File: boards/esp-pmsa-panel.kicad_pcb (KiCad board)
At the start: 2 copper layers, 60 x 120 mm, 183 parts, among them M1 PMSA003, U1 WeMos_D1_mini_Labels, U2 BME68x, U3 OPT3001DNPT

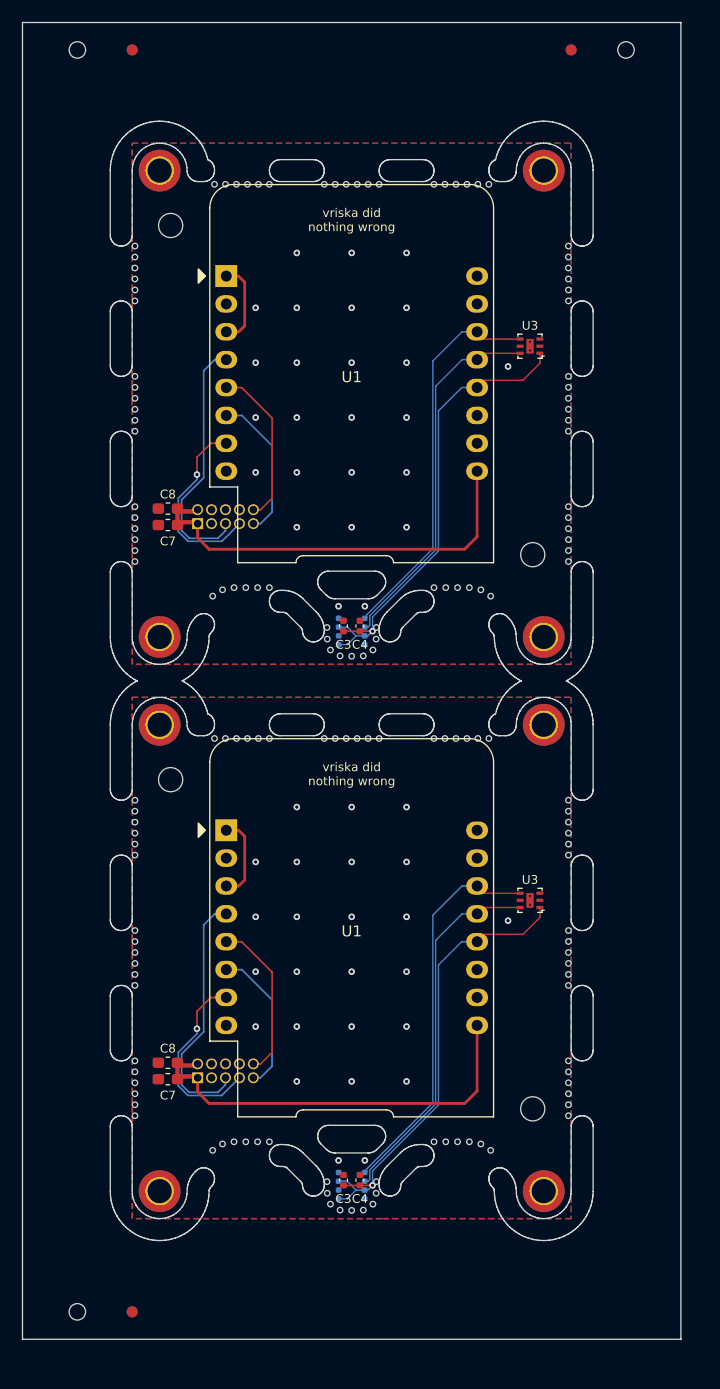
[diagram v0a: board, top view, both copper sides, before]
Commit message: Deploying to gh-pages from @ neg2led/esp-pmsa@e03a36f01e21f29b520752c6169685313d9a0f2f 🚀
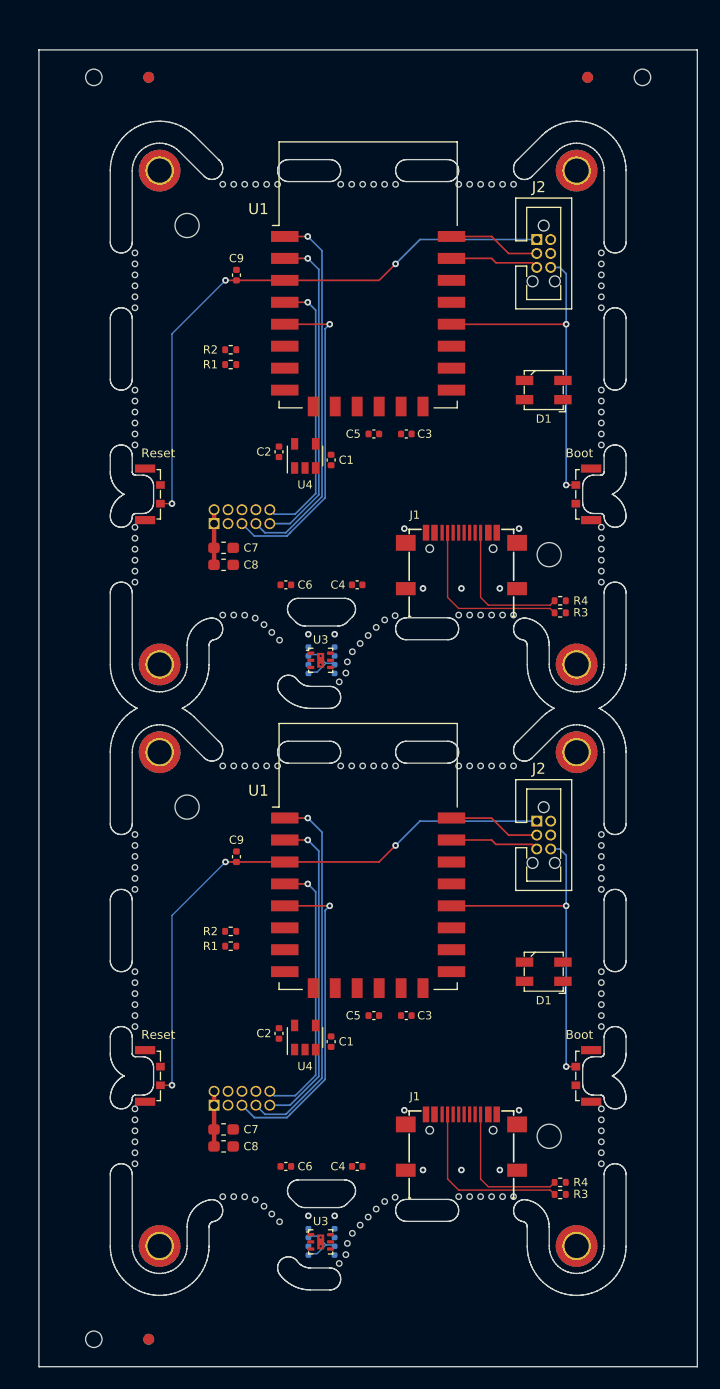
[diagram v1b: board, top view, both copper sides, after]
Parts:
- removed the C3 at (69.3, 144.5)
- removed the C3 at (69.3, 94.0)
- removed the C4 at (70.8, 144.5)
- removed the C4 at (70.8, 94.0)
- removed the C7 at (53.3, 135.3)
- removed the C7 at (53.3, 84.8)
- removed the C8 at (53.3, 133.8)
- removed the C8 at (53.3, 83.3)
- removed the H2 at (87.5, 145.5)
- removed the H2 at (87.5, 95.0)
- removed the H3 at (87.5, 103.0)
- removed the H3 at (87.5, 52.5)
- removed the H4 at (52.5, 145.5)
- removed the H4 at (52.5, 95.0)
- removed the M1 at (70.0, 123.0)
- removed the M1 at (70.0, 72.5)
- removed the REF** at (89.8, 138.6)
- removed the REF** at (89.8, 123.8)
- removed the REF** at (72.5, 104.3)
- removed the REF** at (71.5, 104.3)
- removed the REF** at (70.5, 104.3)
- removed the REF** at (69.5, 104.3)
- removed the REF** at (68.5, 104.3)
- removed the REF** at (67.5, 104.3)
- removed the REF** at (62.5, 104.3)
- removed the REF** at (61.5, 104.3)
- removed the REF** at (60.5, 104.3)
- removed the REF** at (59.5, 104.3)
- removed the REF** at (89.8, 122.8)
- removed the REF** at (58.5, 104.3)
- removed the REF** at (57.5, 104.3)
- removed the REF** at (77.5, 90.5)
- removed the REF** at (78.6, 90.5)
- removed the REF** at (79.6, 90.5)
- removed the REF** at (80.7, 90.5)
- removed the REF** at (81.8, 90.7)
- removed the REF** at (82.7, 91.3)
- removed the REF** at (67.7, 94.1)
- removed the REF** at (67.8, 95.2)
- removed the REF** at (89.8, 121.8)
- removed the REF** at (68.1, 96.2)
- removed the REF** at (68.9, 96.7)
- removed the REF** at (70.0, 96.8)
- removed the REF** at (71.1, 96.7)
- removed the REF** at (71.9, 96.2)
- removed the REF** at (72.2, 95.2)
- removed the REF** at (72.3, 94.1)
- removed the REF** at (57.3, 91.3)
- removed the REF** at (58.2, 90.7)
- removed the REF** at (59.3, 90.5)
- removed the REF** at (89.8, 114.9)
- removed the REF** at (60.4, 90.5)
- removed the REF** at (61.4, 90.5)
- removed the REF** at (62.5, 90.5)
- removed the REF** at (82.5, 53.7)
- removed the REF** at (81.5, 53.7)
- removed the REF** at (80.5, 53.7)
- removed the REF** at (79.5, 53.7)
- removed the REF** at (78.5, 53.7)
- removed the REF** at (77.5, 53.7)
- removed the REF** at (72.5, 53.7)
- removed the REF** at (89.8, 113.9)
- removed the REF** at (71.5, 53.7)
- removed the REF** at (70.5, 53.7)
- removed the REF** at (69.5, 53.7)
- removed the REF** at (68.5, 53.7)
- removed the REF** at (67.5, 53.7)
- removed the REF** at (62.5, 53.7)
- removed the REF** at (61.5, 53.7)
- removed the REF** at (60.5, 53.7)
- removed the REF** at (59.5, 53.7)
- removed the REF** at (58.5, 53.7)
- removed the REF** at (89.8, 112.9)
- removed the REF** at (57.5, 53.7)
- removed the REF** at (45.0, 156.5)
- removed the REF** at (95.0, 41.5)
- removed the REF** at (45.0, 41.5)
- removed the REF** at (50.0, 156.5) (x2)
- removed the REF** at (90.0, 41.5) (x2)
- removed the REF** at (50.0, 41.5) (x2)
- removed the REF** at (89.8, 111.9)
- removed the REF** at (89.8, 110.9)
- removed the REF** at (89.8, 109.9)
- removed the REF** at (50.2, 133.6)
- removed the REF** at (89.8, 137.6)
- removed the REF** at (50.2, 134.6)
- removed the REF** at (50.2, 135.6)
- removed the REF** at (50.2, 136.6)
- removed the REF** at (50.2, 137.6)
- removed the REF** at (50.2, 138.6)
- removed the REF** at (50.2, 121.8)
- removed the REF** at (50.2, 122.8)
- removed the REF** at (50.2, 123.8)
- removed the REF** at (50.2, 124.8)
- removed the REF** at (50.2, 125.8)
- removed the REF** at (89.8, 136.6)
- removed the REF** at (50.2, 126.8)
- removed the REF** at (50.2, 109.9)
- removed the REF** at (50.2, 110.9)
- removed the REF** at (50.2, 111.9)
- removed the REF** at (50.2, 112.9)
- removed the REF** at (50.2, 113.9)
- removed the REF** at (50.2, 114.9)
- removed the REF** at (89.8, 88.1)
- removed the REF** at (89.8, 87.1)
- removed the REF** at (89.8, 86.1)
- removed the REF** at (89.8, 135.6)
- removed the REF** at (89.8, 85.1)
- removed the REF** at (89.8, 84.1)
- removed the REF** at (89.8, 83.1)
- removed the REF** at (89.8, 76.3)
- removed the REF** at (89.8, 75.3)
- removed the REF** at (89.8, 74.3)
- removed the REF** at (89.8, 73.3)
- removed the REF** at (89.8, 72.3)
- removed the REF** at (89.8, 71.3)
- removed the REF** at (89.8, 64.4)
- removed the REF** at (89.8, 134.6)
- removed the REF** at (89.8, 63.4)
- removed the REF** at (89.8, 62.4)
- removed the REF** at (89.8, 61.4)
- removed the REF** at (89.8, 60.4)
- removed the REF** at (89.8, 59.4)
- removed the REF** at (50.2, 83.1)
- removed the REF** at (50.2, 84.1)
- removed the REF** at (50.2, 85.1)
- removed the REF** at (50.2, 86.1)
- removed the REF** at (50.2, 87.1)
- removed the REF** at (89.8, 133.6)
- removed the REF** at (50.2, 88.1)
- removed the REF** at (50.2, 71.3)
- removed the REF** at (50.2, 72.3)
- removed the REF** at (50.2, 73.3)
- removed the REF** at (50.2, 74.3)
- removed the REF** at (50.2, 75.3)
- removed the REF** at (50.2, 76.3)
- removed the REF** at (50.2, 59.4)
- removed the REF** at (50.2, 60.4)
- removed the REF** at (50.2, 61.4)
- removed the REF** at (89.8, 126.8)
- removed the REF** at (50.2, 62.4)
- removed the REF** at (50.2, 63.4)
- removed the REF** at (50.2, 64.4)
- removed the REF** at (77.5, 141.0)
- removed the REF** at (78.6, 141.0)
- removed the REF** at (79.6, 141.0)
- removed the REF** at (80.7, 141.0)
- removed the REF** at (81.8, 141.2)
- removed the REF** at (82.7, 141.8)
- removed the REF** at (67.7, 144.6)
- removed the REF** at (89.8, 125.8)
- removed the REF** at (67.8, 145.7)
- removed the REF** at (68.1, 146.7)
- removed the REF** at (68.9, 147.2)
- removed the REF** at (70.0, 147.3)
- removed the REF** at (71.1, 147.2)
- removed the REF** at (71.9, 146.7)
- removed the REF** at (72.2, 145.7)
- removed the REF** at (72.3, 144.6)
- removed the REF** at (57.3, 141.8)
- removed the REF** at (58.2, 141.2)
- removed the REF** at (89.8, 124.8)
- removed the REF** at (59.3, 141.0)
- removed the REF** at (60.4, 141.0)
- removed the REF** at (61.4, 141.0)
- removed the REF** at (62.5, 141.0)
- removed the REF** at (82.5, 104.3)
- removed the REF** at (81.5, 104.3)
- removed the REF** at (80.5, 104.3)
- removed the REF** at (79.5, 104.3)
- removed the REF** at (78.5, 104.3)
- removed the REF** at (77.5, 104.3)
- removed the U1 at (70.0, 121.5)
- removed the U1 at (70.0, 71.0)
- removed the U2 at (70.0, 145.0)
- removed the U2 at (70.0, 94.5)
- removed the U3 at (86.3, 119.0)
- removed the U3 at (86.3, 68.5)
- added C1: 10u, Capacitor_SMD:C_0402_1005Metric, F.Cu at (68.1, 131.9)
- added C1: 10u, Capacitor_SMD:C_0402_1005Metric, F.Cu at (68.1, 78.9)
- added C2: 10u, Capacitor_SMD:C_0402_1005Metric, F.Cu at (63.4, 131.1)
- added C2: 10u, Capacitor_SMD:C_0402_1005Metric, F.Cu at (63.4, 78.1)
- added C3: 1u, Capacitor_SMD:C_0402_1005Metric, F.Cu at (75.0, 129.5)
- added C3: 1u, Capacitor_SMD:C_0402_1005Metric, F.Cu at (75.0, 76.5)
- added C4: 0.1u, Capacitor_SMD:C_0402_1005Metric, F.Cu at (70.5, 143.3)
- added C4: 0.1u, Capacitor_SMD:C_0402_1005Metric, F.Cu at (70.5, 90.3)
- added C5: 1u, Capacitor_SMD:C_0402_1005Metric, F.Cu at (72.0, 129.5)
- added C5: 1u, Capacitor_SMD:C_0402_1005Metric, F.Cu at (72.0, 76.5)
- added C6: 0.1u, Capacitor_SMD:C_0402_1005Metric, F.Cu at (64.0, 143.3)
- added C6: 0.1u, Capacitor_SMD:C_0402_1005Metric, F.Cu at (64.0, 90.3)
- added C7: 10u, Capacitor_SMD:C_0603_1608Metric_Pad1.05x0.95mm_HandSolder, F.Cu at (58.3, 139.9)
- added C7: 10u, Capacitor_SMD:C_0603_1608Metric_Pad1.05x0.95mm_HandSolder, F.Cu at (58.3, 86.9)
- added C8: 10u, Capacitor_SMD:C_0603_1608Metric_Pad1.05x0.95mm_HandSolder, F.Cu at (58.3, 141.4)
- added C8: 10u, Capacitor_SMD:C_0603_1608Metric_Pad1.05x0.95mm_HandSolder, F.Cu at (58.3, 88.4)
- added C9: 0.1u, Capacitor_SMD:C_0402_1005Metric, F.Cu at (59.5, 115.0)
- added C9: 0.1u, Capacitor_SMD:C_0402_1005Metric, F.Cu at (59.5, 62.0)
- added D1: APA104-12-3535, 21-SnapEDA-zip:LED_APA104-12-3535, F.Cu at (87.5, 125.5)
- added D1: APA104-12-3535, 21-SnapEDA-zip:LED_APA104-12-3535, F.Cu at (87.5, 72.5)
- added H2: MP, MountingHole:MountingHole_2.2mm_M2_DIN965_Pad_TopBottom, F.Cu at (90.5, 150.5)
- added H2: MP, MountingHole:MountingHole_2.2mm_M2_DIN965_Pad_TopBottom, F.Cu at (90.5, 97.5)
- added H3: MP, MountingHole:MountingHole_2.2mm_M2_DIN965_Pad_TopBottom, F.Cu at (90.5, 105.5)
- added H3: MP, MountingHole:MountingHole_2.2mm_M2_DIN965_Pad_TopBottom, F.Cu at (90.5, 52.5)
- added H4: MP, MountingHole:MountingHole_2.2mm_M2_DIN965_Pad_TopBottom, F.Cu at (52.5, 150.5)
- added H4: MP, MountingHole:MountingHole_2.2mm_M2_DIN965_Pad_TopBottom, F.Cu at (52.5, 97.5)
- added J1: USB_C_Receptacle_USB2.0_304S-ACP16, 41-EasyEDA-Edits:USB-C-SMD_TYPEC-304S-ACP16, F.Cu at (80.0, 141.1)
- added J1: USB_C_Receptacle_USB2.0_304S-ACP16, 41-EasyEDA-Edits:USB-C-SMD_TYPEC-304S-ACP16, F.Cu at (80.0, 88.1)
- added J2: ESP-PROG, 11-My-Edits:TC2030_IDCBox_2x03_P1.25mm_Vertical_3D, F.Cu at (87.5, 113.1)
- added J2: ESP-PROG, 11-My-Edits:TC2030_IDCBox_2x03_P1.25mm_Vertical_3D, F.Cu at (87.5, 60.1)
- added M1: PMSA003, 12-Collected-Footprints:PMSA003, B.Cu at (71.5, 125.5)
- added M1: PMSA003, 12-Collected-Footprints:PMSA003, B.Cu at (71.5, 72.5)
- added R1: 4k7, Resistor_SMD:R_0402_1005Metric, F.Cu at (59.0, 123.2)
- added R1: 4k7, Resistor_SMD:R_0402_1005Metric, F.Cu at (59.0, 70.2)
- added R2: 4k7, Resistor_SMD:R_0402_1005Metric, F.Cu at (59.0, 121.8)
- added R2: 4k7, Resistor_SMD:R_0402_1005Metric, F.Cu at (59.0, 68.8)
- added R3: 5k1, Resistor_SMD:R_0402_1005Metric, F.Cu at (89.0, 145.8)
- added R3: 5k1, Resistor_SMD:R_0402_1005Metric, F.Cu at (89.0, 92.8)
- added R4: 5k1, Resistor_SMD:R_0402_1005Metric, F.Cu at (89.0, 144.7)
- added R4: 5k1, Resistor_SMD:R_0402_1005Metric, F.Cu at (89.0, 91.7)
- added REF**: NPTH, NPTH, F.Cu at (92.8, 143.0)
- added REF**: NPTH, NPTH, F.Cu at (92.8, 127.5)
- added REF**: NPTH, NPTH, F.Cu at (79.8, 106.8)
- added REF**: NPTH, NPTH, F.Cu at (74.0, 106.8)
- added REF**: NPTH, NPTH, F.Cu at (73.0, 106.8)
- added REF**: NPTH, NPTH, F.Cu at (72.0, 106.8)
- added REF**: NPTH, NPTH, F.Cu at (71.0, 106.8)
- added REF**: NPTH, NPTH, F.Cu at (70.0, 106.8)
- added REF**: NPTH, NPTH, F.Cu at (69.0, 106.8)
- added REF**: NPTH, NPTH, F.Cu at (63.3, 106.8)
- added REF**: NPTH, NPTH, F.Cu at (62.3, 106.8)
- added REF**: NPTH, NPTH, F.Cu at (61.3, 106.8)
- added REF**: NPTH, NPTH, F.Cu at (92.8, 126.5)
- added REF**: NPTH, NPTH, F.Cu at (60.3, 106.8)
- added REF**: NPTH, NPTH, F.Cu at (59.3, 106.8)
- added REF**: NPTH, NPTH, F.Cu at (58.3, 106.8)
- added REF**: NPTH, NPTH, F.Cu at (79.8, 93.0)
- added REF**: NPTH, NPTH, F.Cu at (80.8, 93.0)
- added REF**: NPTH, NPTH, F.Cu at (81.8, 93.0)
- added REF**: NPTH, NPTH, F.Cu at (82.8, 93.0)
- added REF**: NPTH, NPTH, F.Cu at (83.8, 93.0)
- added REF**: NPTH, NPTH, F.Cu at (84.8, 93.0)
- added REF**: NPTH, NPTH, F.Cu at (68.9, 99.1)
- added REF**: NPTH, NPTH, F.Cu at (92.8, 125.5)
- added REF**: NPTH, NPTH, F.Cu at (69.5, 98.3)
- added REF**: NPTH, NPTH, F.Cu at (69.6, 97.3)
- added REF**: NPTH, NPTH, F.Cu at (70.1, 96.3)
- added REF**: NPTH, NPTH, F.Cu at (70.8, 95.6)
- added REF**: NPTH, NPTH, F.Cu at (71.5, 94.9)
- added REF**: NPTH, NPTH, F.Cu at (72.2, 94.1)
- added REF**: NPTH, NPTH, F.Cu at (73.0, 93.4)
- added REF**: NPTH, NPTH, F.Cu at (74.0, 93.1)
- added REF**: NPTH, NPTH, F.Cu at (58.3, 93.0)
- added REF**: NPTH, NPTH, F.Cu at (59.3, 93.0)
- added REF**: NPTH, NPTH, F.Cu at (92.8, 118.0)
- added REF**: NPTH, NPTH, F.Cu at (60.3, 93.0)
- added REF**: NPTH, NPTH, F.Cu at (61.2, 93.3)
- added REF**: NPTH, NPTH, F.Cu at (62.0, 93.9)
- added REF**: NPTH, NPTH, F.Cu at (62.7, 94.6)
- added REF**: NPTH, NPTH, F.Cu at (63.4, 95.3)
- added REF**: NPTH, NPTH, F.Cu at (84.8, 53.7)
- added REF**: NPTH, NPTH, F.Cu at (83.8, 53.7)
- added REF**: NPTH, NPTH, F.Cu at (82.8, 53.7)
- added REF**: NPTH, NPTH, F.Cu at (81.8, 53.7)
- added REF**: NPTH, NPTH, F.Cu at (80.8, 53.7)
- added REF**: NPTH, NPTH, F.Cu at (92.8, 117.0)
- added REF**: NPTH, NPTH, F.Cu at (79.8, 53.7)
- added REF**: NPTH, NPTH, F.Cu at (74.0, 53.7)
- added REF**: NPTH, NPTH, F.Cu at (73.0, 53.7)
- added REF**: NPTH, NPTH, F.Cu at (72.0, 53.7)
- added REF**: NPTH, NPTH, F.Cu at (71.0, 53.7)
- added REF**: NPTH, NPTH, F.Cu at (70.0, 53.7)
- added REF**: NPTH, NPTH, F.Cu at (69.0, 53.7)
- added REF**: NPTH, NPTH, F.Cu at (63.3, 53.7)
- added REF**: NPTH, NPTH, F.Cu at (62.3, 53.7)
- added REF**: NPTH, NPTH, F.Cu at (61.3, 53.7)
- added REF**: NPTH, NPTH, F.Cu at (92.8, 116.0)
- added REF**: NPTH, NPTH, F.Cu at (60.3, 53.7)
- added REF**: NPTH, NPTH, F.Cu at (59.3, 53.7)
- added REF**: NPTH, NPTH, F.Cu at (58.3, 53.7)
- added REF**: NPTH, NPTH, F.Cu at (46.5, 159.0)
- added REF**: NPTH, NPTH, F.Cu at (96.5, 44.0)
- added REF**: NPTH, NPTH, F.Cu at (46.5, 44.0)
- added REF**: Fiducial, Fiducial, B.Cu at (51.5, 159.0)
- added REF**: Fiducial, Fiducial, F.Cu at (51.5, 159.0)
- added REF**: Fiducial, Fiducial, B.Cu at (91.5, 44.0)
- added REF**: Fiducial, Fiducial, F.Cu at (91.5, 44.0)
- added REF**: NPTH, NPTH, F.Cu at (92.8, 115.0)
- added REF**: Fiducial, Fiducial, B.Cu at (51.5, 44.0)
- added REF**: Fiducial, Fiducial, F.Cu at (51.5, 44.0)
- added REF**: NPTH, NPTH, F.Cu at (92.8, 114.0)
- added REF**: NPTH, NPTH, F.Cu at (92.8, 113.0)
- added REF**: NPTH, NPTH, F.Cu at (50.2, 138.0)
- added REF**: NPTH, NPTH, F.Cu at (92.8, 142.0)
- added REF**: NPTH, NPTH, F.Cu at (50.2, 139.0)
- added REF**: NPTH, NPTH, F.Cu at (50.2, 140.0)
- added REF**: NPTH, NPTH, F.Cu at (50.2, 141.0)
- added REF**: NPTH, NPTH, F.Cu at (50.2, 142.0)
- added REF**: NPTH, NPTH, F.Cu at (50.2, 143.0)
- added REF**: NPTH, NPTH, F.Cu at (50.2, 125.5)
- added REF**: NPTH, NPTH, F.Cu at (50.2, 126.5)
- added REF**: NPTH, NPTH, F.Cu at (50.2, 127.5)
- added REF**: NPTH, NPTH, F.Cu at (50.2, 128.5)
- added REF**: NPTH, NPTH, F.Cu at (50.2, 129.5)
- added REF**: NPTH, NPTH, F.Cu at (92.8, 141.0)
- added REF**: NPTH, NPTH, F.Cu at (50.2, 130.5)
- added REF**: NPTH, NPTH, F.Cu at (50.2, 113.0)
- added REF**: NPTH, NPTH, F.Cu at (50.2, 114.0)
- added REF**: NPTH, NPTH, F.Cu at (50.2, 115.0)
- added REF**: NPTH, NPTH, F.Cu at (50.2, 116.0)
- added REF**: NPTH, NPTH, F.Cu at (50.2, 117.0)
- added REF**: NPTH, NPTH, F.Cu at (50.2, 118.0)
- added REF**: NPTH, NPTH, F.Cu at (92.8, 90.0)
- added REF**: NPTH, NPTH, F.Cu at (92.8, 89.0)
- added REF**: NPTH, NPTH, F.Cu at (92.8, 88.0)
- added REF**: NPTH, NPTH, F.Cu at (92.8, 140.0)
- added REF**: NPTH, NPTH, F.Cu at (92.8, 87.0)
- added REF**: NPTH, NPTH, F.Cu at (92.8, 86.0)
- added REF**: NPTH, NPTH, F.Cu at (92.8, 85.0)
- added REF**: NPTH, NPTH, F.Cu at (92.8, 77.5)
- added REF**: NPTH, NPTH, F.Cu at (92.8, 76.5)
- added REF**: NPTH, NPTH, F.Cu at (92.8, 75.5)
- added REF**: NPTH, NPTH, F.Cu at (92.8, 74.5)
- added REF**: NPTH, NPTH, F.Cu at (92.8, 73.5)
- added REF**: NPTH, NPTH, F.Cu at (92.8, 72.5)
- added REF**: NPTH, NPTH, F.Cu at (92.8, 65.0)
- added REF**: NPTH, NPTH, F.Cu at (92.8, 139.0)
- added REF**: NPTH, NPTH, F.Cu at (92.8, 64.0)
- added REF**: NPTH, NPTH, F.Cu at (92.8, 63.0)
- added REF**: NPTH, NPTH, F.Cu at (92.8, 62.0)
- added REF**: NPTH, NPTH, F.Cu at (92.8, 61.0)
- added REF**: NPTH, NPTH, F.Cu at (92.8, 60.0)
- added REF**: NPTH, NPTH, F.Cu at (50.2, 85.0)
- added REF**: NPTH, NPTH, F.Cu at (50.2, 86.0)
- added REF**: NPTH, NPTH, F.Cu at (50.2, 87.0)
- added REF**: NPTH, NPTH, F.Cu at (50.2, 88.0)
- added REF**: NPTH, NPTH, F.Cu at (50.2, 89.0)
- added REF**: NPTH, NPTH, F.Cu at (92.8, 138.0)
- added REF**: NPTH, NPTH, F.Cu at (50.2, 90.0)
- added REF**: NPTH, NPTH, F.Cu at (50.2, 72.5)
- added REF**: NPTH, NPTH, F.Cu at (50.2, 73.5)
- added REF**: NPTH, NPTH, F.Cu at (50.2, 74.5)
- added REF**: NPTH, NPTH, F.Cu at (50.2, 75.5)
- added REF**: NPTH, NPTH, F.Cu at (50.2, 76.5)
- added REF**: NPTH, NPTH, F.Cu at (50.2, 77.5)
- added REF**: NPTH, NPTH, F.Cu at (50.2, 60.0)
- added REF**: NPTH, NPTH, F.Cu at (50.2, 61.0)
- added REF**: NPTH, NPTH, F.Cu at (50.2, 62.0)
- added REF**: NPTH, NPTH, F.Cu at (92.8, 130.5)
- added REF**: NPTH, NPTH, F.Cu at (50.2, 63.0)
- added REF**: NPTH, NPTH, F.Cu at (50.2, 64.0)
- added REF**: NPTH, NPTH, F.Cu at (50.2, 65.0)
- added REF**: NPTH, NPTH, F.Cu at (79.8, 146.0)
- added REF**: NPTH, NPTH, F.Cu at (80.8, 146.0)
- added REF**: NPTH, NPTH, F.Cu at (81.8, 146.0)
- added REF**: NPTH, NPTH, F.Cu at (82.8, 146.0)
- added REF**: NPTH, NPTH, F.Cu at (83.8, 146.0)
- added REF**: NPTH, NPTH, F.Cu at (84.8, 146.0)
- added REF**: NPTH, NPTH, F.Cu at (68.9, 152.1)
- added REF**: NPTH, NPTH, F.Cu at (92.8, 129.5)
- added REF**: NPTH, NPTH, F.Cu at (69.5, 151.3)
- added REF**: NPTH, NPTH, F.Cu at (69.6, 150.3)
- added REF**: NPTH, NPTH, F.Cu at (70.1, 149.3)
- added REF**: NPTH, NPTH, F.Cu at (70.8, 148.6)
- added REF**: NPTH, NPTH, F.Cu at (71.5, 147.9)
- added REF**: NPTH, NPTH, F.Cu at (72.2, 147.1)
- added REF**: NPTH, NPTH, F.Cu at (73.0, 146.4)
- added REF**: NPTH, NPTH, F.Cu at (74.0, 146.1)
- added REF**: NPTH, NPTH, F.Cu at (58.3, 146.0)
- added REF**: NPTH, NPTH, F.Cu at (59.3, 146.0)
- added REF**: NPTH, NPTH, F.Cu at (92.8, 128.5)
- added REF**: NPTH, NPTH, F.Cu at (60.3, 146.0)
- added REF**: NPTH, NPTH, F.Cu at (61.2, 146.3)
- added REF**: NPTH, NPTH, F.Cu at (62.0, 146.9)
- added REF**: NPTH, NPTH, F.Cu at (62.7, 147.6)
- added REF**: NPTH, NPTH, F.Cu at (63.4, 148.3)
- added REF**: NPTH, NPTH, F.Cu at (84.8, 106.8)
- added REF**: NPTH, NPTH, F.Cu at (83.8, 106.8)
- added REF**: NPTH, NPTH, F.Cu at (82.8, 106.8)
- added REF**: NPTH, NPTH, F.Cu at (81.8, 106.8)
- added REF**: NPTH, NPTH, F.Cu at (80.8, 106.8)
- added SW1: Reset, 41-EasyEDA-Edits:SW-SMD_SKSLLAE010-3D, F.Cu at (51.9, 135.0)
- added SW1: Reset, 41-EasyEDA-Edits:SW-SMD_SKSLLAE010-3D, F.Cu at (51.9, 82.0)
- added SW2: Boot, 41-EasyEDA-Edits:SW-SMD_SKSLLAE010-3D, F.Cu at (91.1, 135.0)
- added SW2: Boot, 41-EasyEDA-Edits:SW-SMD_SKSLLAE010-3D, F.Cu at (91.1, 82.0)
- added U1: ESP32-C3F, 11-My-Edits:ESP-12H, F.Cu at (71.5, 115.0)
- added U1: ESP32-C3F, 11-My-Edits:ESP-12H, F.Cu at (71.5, 62.0)
- added U2: BME68x, 11-My-Edits:Bosch_LGA-8_3x3mm_P0.8mm_ClockwisePinNumbering, B.Cu at (67.3, 150.1)
- added U2: BME68x, 11-My-Edits:Bosch_LGA-8_3x3mm_P0.8mm_ClockwisePinNumbering, B.Cu at (67.3, 97.1)
- added U3: OPT3001DNPT, 11-My-Edits:MultiALS-LTR303-TIOPT3K, F.Cu at (67.2, 150.1)
- added U3: OPT3001DNPT, 11-My-Edits:MultiALS-LTR303-TIOPT3K, F.Cu at (67.2, 97.1)
- added U4: XC6220B331MR, Package_TO_SOT_SMD:SOT-23-5, F.Cu at (65.8, 131.5)
- added U4: XC6220B331MR, Package_TO_SOT_SMD:SOT-23-5, F.Cu at (65.8, 78.5)
- moved H1 2.50 mm to (52.5, 105.5)
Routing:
- net Board_2-Board_1-/~RST: track 0.00 -> 53.6 mm, vias 0 -> 3
- net Board_1-Board_1-/~RST: track 0.00 -> 53.6 mm, vias 0 -> 3
- net Board_1-Board_1-/VCC_SENS: track 42.8 -> 0.00 mm, vias 1 -> 0
- net Board_2-Board_1-/VCC_SENS: track 42.8 -> 0.00 mm, vias 1 -> 0
- net Board_2-Board_1-/SCL: track 35.5 -> 0.00 mm
- net Board_1-Board_1-/SCL: track 35.5 -> 0.00 mm
- net Board_1-Board_1-+5V: track 39.4 -> 5.03 mm
- net Board_2-Board_1-+5V: track 39.4 -> 5.03 mm
- net Board_1-Board_1-/SDA: track 33.8 -> 0.00 mm
- net Board_2-Board_1-/SDA: track 33.8 -> 0.00 mm
- net Board_2-Board_1-/~BOOT: track 0.00 -> 32.2 mm, vias 0 -> 2
- net Board_1-Board_1-/~BOOT: track 0.00 -> 32.2 mm, vias 0 -> 2
- net Board_1-Board_1-/PMS_RX: track 17.0 -> 34.1 mm
- net Board_2-Board_1-/PMS_RX: track 17.0 -> 34.1 mm
- net Board_1-Board_1-Net-(J1-PadA5): track 0.00 -> 16.2 mm
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- removed copper zone on B.Cu, net Board_1-Board_1-GND
- removed copper zone on F.Cu, net Board_1-Board_1-GND
- removed copper zone on B.Cu, net Board_2-Board_1-GND
- removed copper zone on F.Cu, net Board_2-Board_1-GND
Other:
- outline, holes or cut-outs redrawn
- board text added: "Boot"
- board text added: "Reset"
- board text removed: "vriska did nothing wrong"
